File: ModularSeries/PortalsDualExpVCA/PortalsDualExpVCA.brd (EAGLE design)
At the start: 47 x 95 mm, 71 parts, among them IC1 LM13700_DIP, IC2 TL0X4_DIP, IC3 TL0X4_DIP, Q1 2N3906, Q2 2N3906, Q3 2N3906, Q4 2N3906

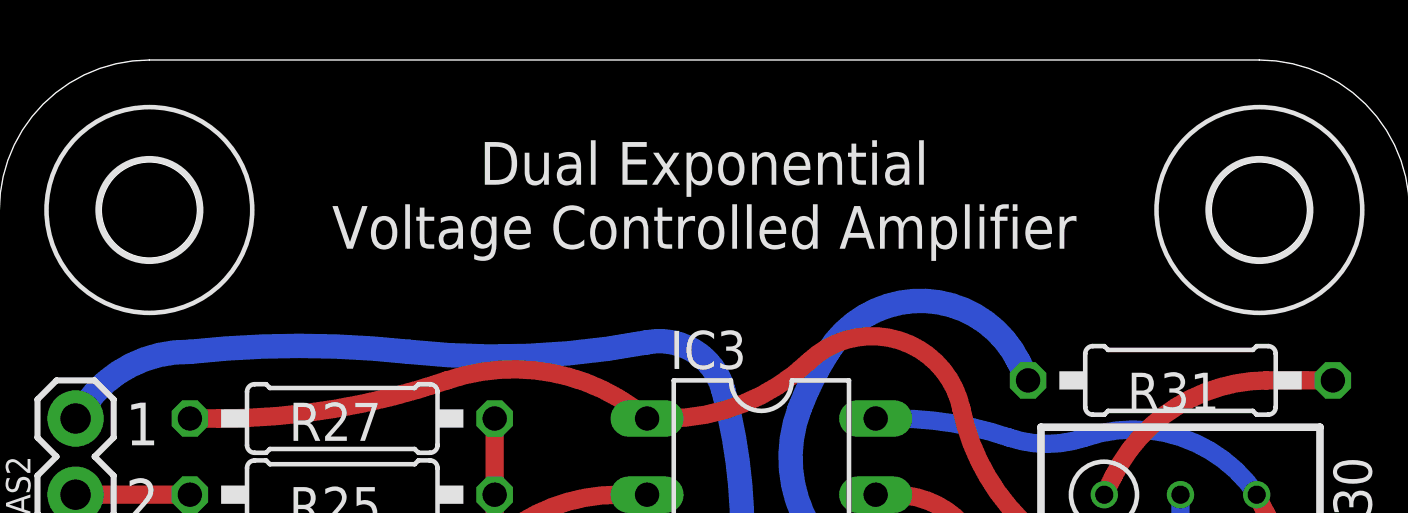
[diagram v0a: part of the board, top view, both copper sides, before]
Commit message: Portals files updated, schematic exports and images included
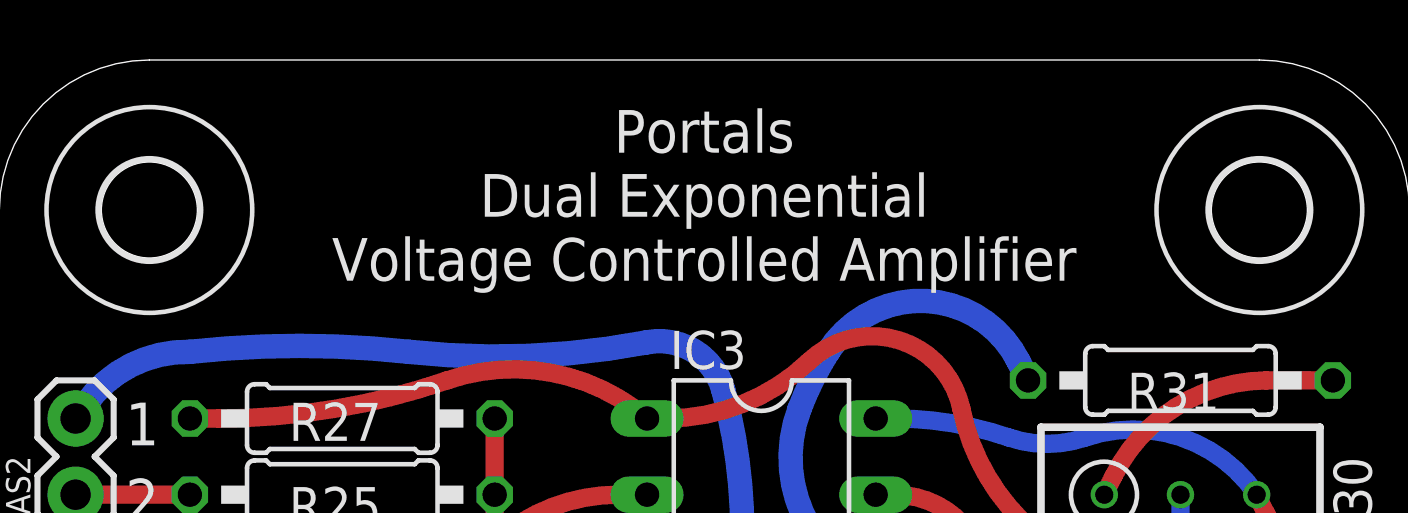
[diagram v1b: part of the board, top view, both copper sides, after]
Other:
- board text added: "Portals Dual Exponential Voltage Controlled Amplifier"
- board text removed: "Dual Exponential Voltage Controlled Amplifier"
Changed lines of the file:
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@@
 <text x="4.7625" y="80.3275" size="1.4224" layer="21" font="vector" ratio="12" align="center">2</text>
 <text x="4.7625" y="82.8675" size="1.4224" layer="21" font="vector" ratio="12" align="center">1</text>
-<text x="23.495" y="90.4875" size="1.4224" layer="21" font="vector" ratio="12" align="center">Dual Exponential
+<text x="23.495" y="90.4875" size="1.4224" layer="21" font="vector" ratio="12" align="center">Portals
+Dual Exponential
 Voltage Controlled Amplifier</text>
 <text x="23.495" y="4.445" size="1.4224" layer="21" font="vector" ratio="12" align="center">v2.0
